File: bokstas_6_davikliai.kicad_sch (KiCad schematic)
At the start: 65 parts, among them J1 Conn_01x10, J2 Conn_01x03, K1.1 Coil, K1.2 RelayContact_NONC, K2.1 Coil, K2.2 RelayContact_NONC, K3.1 Coil, K3.2 RelayContact_NONC, K4.1 Coil, K4.2 RelayContact_NONC, K5.1 Coil, K5.2 RelayContact_NONC, K6.1 Coil, K6.2 RelayContact_NONC, K7 OUT, Q1 BC817, Q2 BC817, U1 L7812, U2 4049, U3 NE555P, X1 Optic1L, X2 Optic2L, X3 Optic3L, X4 Optic1R, X5 Optic2R, X6 Optic3R

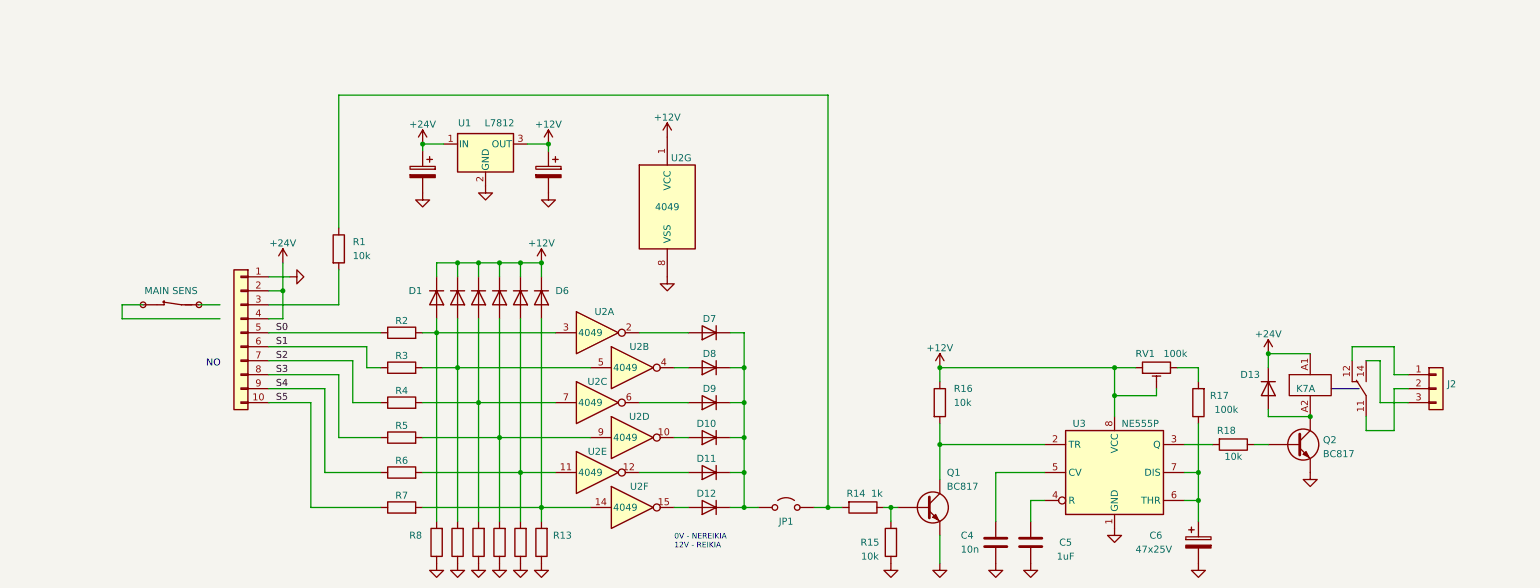
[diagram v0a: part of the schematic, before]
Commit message: versija 1.0
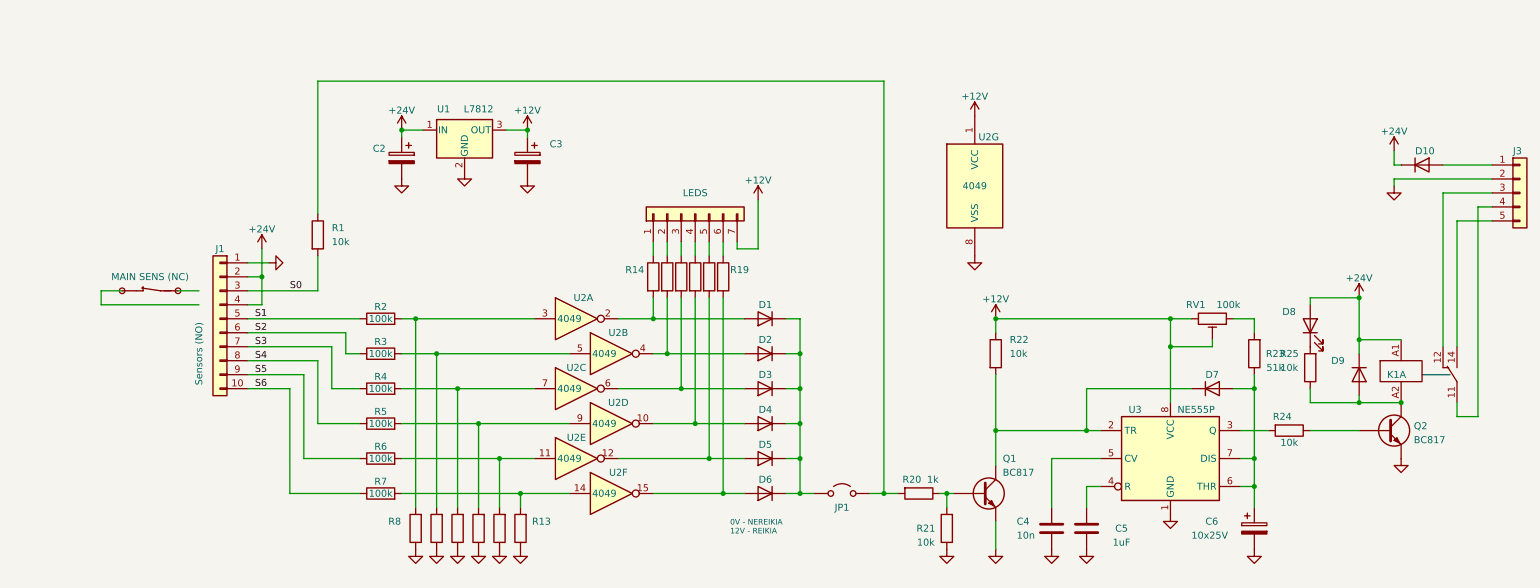
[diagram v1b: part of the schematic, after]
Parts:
- removed D1, D2, D3, D4, D5, D6: BAS32, Diode_SMD:D_MiniMELF, symbol Device:D
- removed J2: Conn_01x03, symbol Connector_Generic:Conn_01x03
- added D10: LL4007, Diode_SMD:D_MELF, symbol Device:D
- added D7: BAS32, Diode_SMD:D_MiniMELF, symbol Device:D
- added D8: LED, LED_THT:LED_D3.0mm, symbol Device:LED
- added J2: LEDS, Connector_PinHeader_2.54mm:PinHeader_1x07_P2.54mm_Vertical, symbol Connector_Generic:Conn_01x07
- added J3: Conn_01x05, Connector_PinHeader_2.54mm:PinHeader_1x05_P2.54mm_Vertical, symbol Connector_Generic:Conn_01x05
- added R14, R15, R16, R17, R18, R19: 10k, Resistor_THT:R_Axial_DIN0204_L3.6mm_D1.6mm_P7.62mm_Horizontal, symbol Device:R
- added R25: 10k, Resistor_SMD:R_0805_2012Metric, symbol Device:R
- C1: value MAIN SENS -> MAIN SENS (NC)
- C2: value C_Polarized -> 100x35V; footprint (none) -> Capacitor_THT:CP_Radial_D8.0mm_P2.50mm
- C3: value C_Polarized -> 330x16V; footprint (none) -> Capacitor_THT:CP_Radial_D8.0mm_P2.50mm
- C6: value 47x25V -> 10x25V
- J1: value Conn_01x10 -> Sensors (NO); footprint (none) -> Connector_PinHeader_2.54mm:PinHeader_1x10_P2.54mm_Vertical
- R1: footprint Resistor_SMD:R_0805_2012Metric -> Resistor_THT:R_Axial_DIN0204_L3.6mm_D1.6mm_P7.62mm_Horizontal
- R2, R3, R4, R5, R6, R7: value R -> 100k; footprint Resistor_SMD:R_0805_2012Metric -> Resistor_THT:R_Axial_DIN0204_L3.6mm_D1.6mm_P7.62mm_Horizontal
- R23: renamed from R17; value 100k -> 51k
- U2: footprint Package_DIP:DIP-14_W7.62mm -> Package_DIP:DIP-16_W7.62mm
- renumbered D7 to D1, D8 to D2, D9 to D3, D10 to D4, D11 to D5, D12 to D6, D13 to D9, K7 to K1, R14 to R20, R15 to R21, R16 to R22, R18 to R24
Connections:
- net +12V: now also RV1.3, J2.7 (Pin_7); no longer RV1.1
- net +24V: now also D10.1 (K), D8.2 (A)
- net GND: now also J3.2 (Pin_2)
- net S0: now also J1.3 (Pin_3), R1.2; no longer J1.5 (Pin_5), R2.1
- net S1: now also J1.5 (Pin_5), R2.1; no longer J1.6 (Pin_6), R3.1
- net S2: now also J1.6 (Pin_6), R3.1; no longer J1.7 (Pin_7), R4.1
- net S3: now also J1.7 (Pin_7), R4.1; no longer J1.8 (Pin_8), R5.1
- net S4: now also J1.8 (Pin_8), R5.1; no longer J1.9 (Pin_9), R6.1
- net S5: now also J1.9 (Pin_9), R6.1; no longer J1.10 (Pin_10), R7.1
- net at D2.2 (A), U2.4: now also R15.2
- net at D1.2 (A), U2.2: now also R14.2
- net at C6.1, R23.1, U3.6 (THR)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: now also D7.2 (A)
- net at R23.2: now also RV1.1; no longer RV1.3
- net at D9.2 (A), K1.A2, Q2.3 (C): now also R25.1
- net at D4.2 (A), U2.10: now also R17.2
- net at K1.12: now also J3.3 (Pin_3)
- net at K1.11: now also J3.4 (Pin_4)
- net at K1.14: now also J3.5 (Pin_5)
- net at D3.2 (A), U2.6: now also R16.2
- net at Q1.3 (C), R22.2, U3.2 (TR): now also D7.1 (K)
- net at D5.2 (A), U2.12: now also R18.2
- net at D6.2 (A), U2.15: now also R19.2
- new net: J2.6 (Pin_6), R19.1
- new net: D10.2 (A), J3.1 (Pin_1)
- new net: J2.2 (Pin_2), R15.1
- new net: J2.4 (Pin_4), R17.1
- new net: D8.1 (K), R25.2
- new net: J2.1 (Pin_1), R14.1
- new net: J2.3 (Pin_3), R16.1
- new net: J2.5 (Pin_5), R18.1
- new net S6: J1.10 (Pin_10), R7.1
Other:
- moved on the sheet: C4, C5, C6, D1, D2, D3, D4, D5, D6, D9, JP1, K1A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
